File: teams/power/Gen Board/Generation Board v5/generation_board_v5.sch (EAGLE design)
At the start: 210 parts, among them U2 LT3652, U3 LT3652, U4 LT3652, U5 TPS732XX, U7 TPS732XX

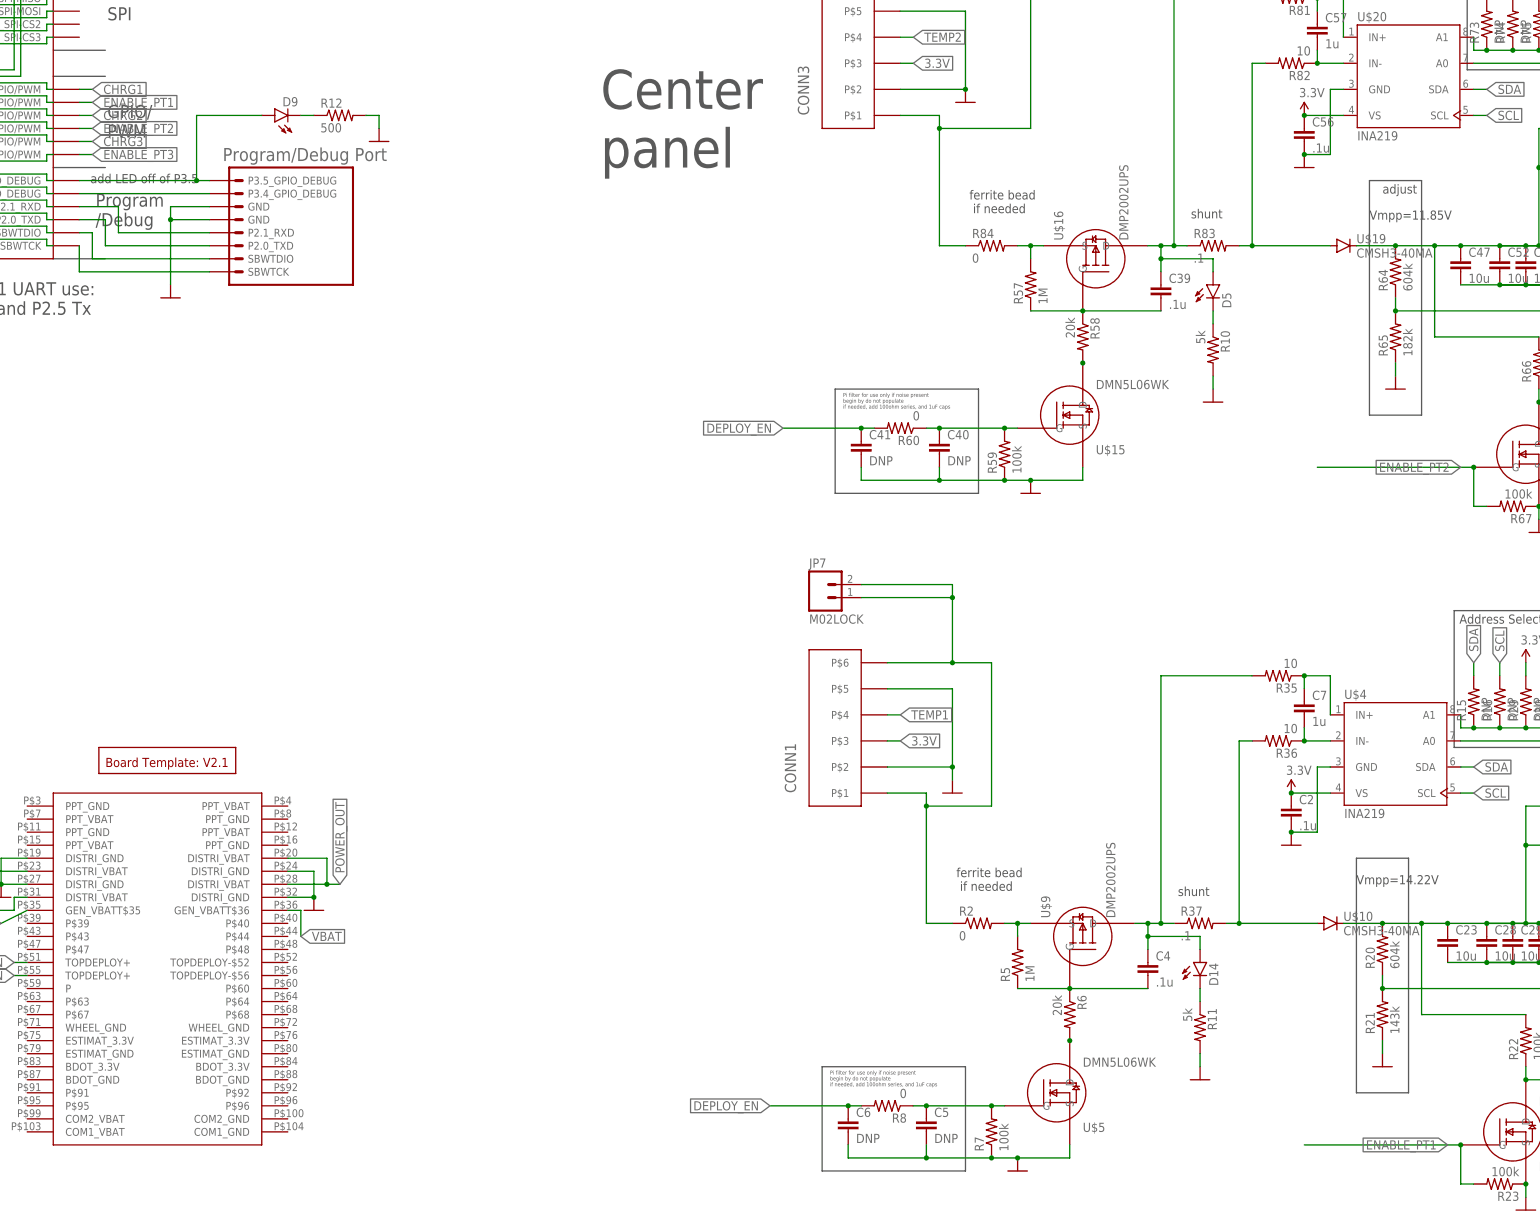
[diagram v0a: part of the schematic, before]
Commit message: minor changes
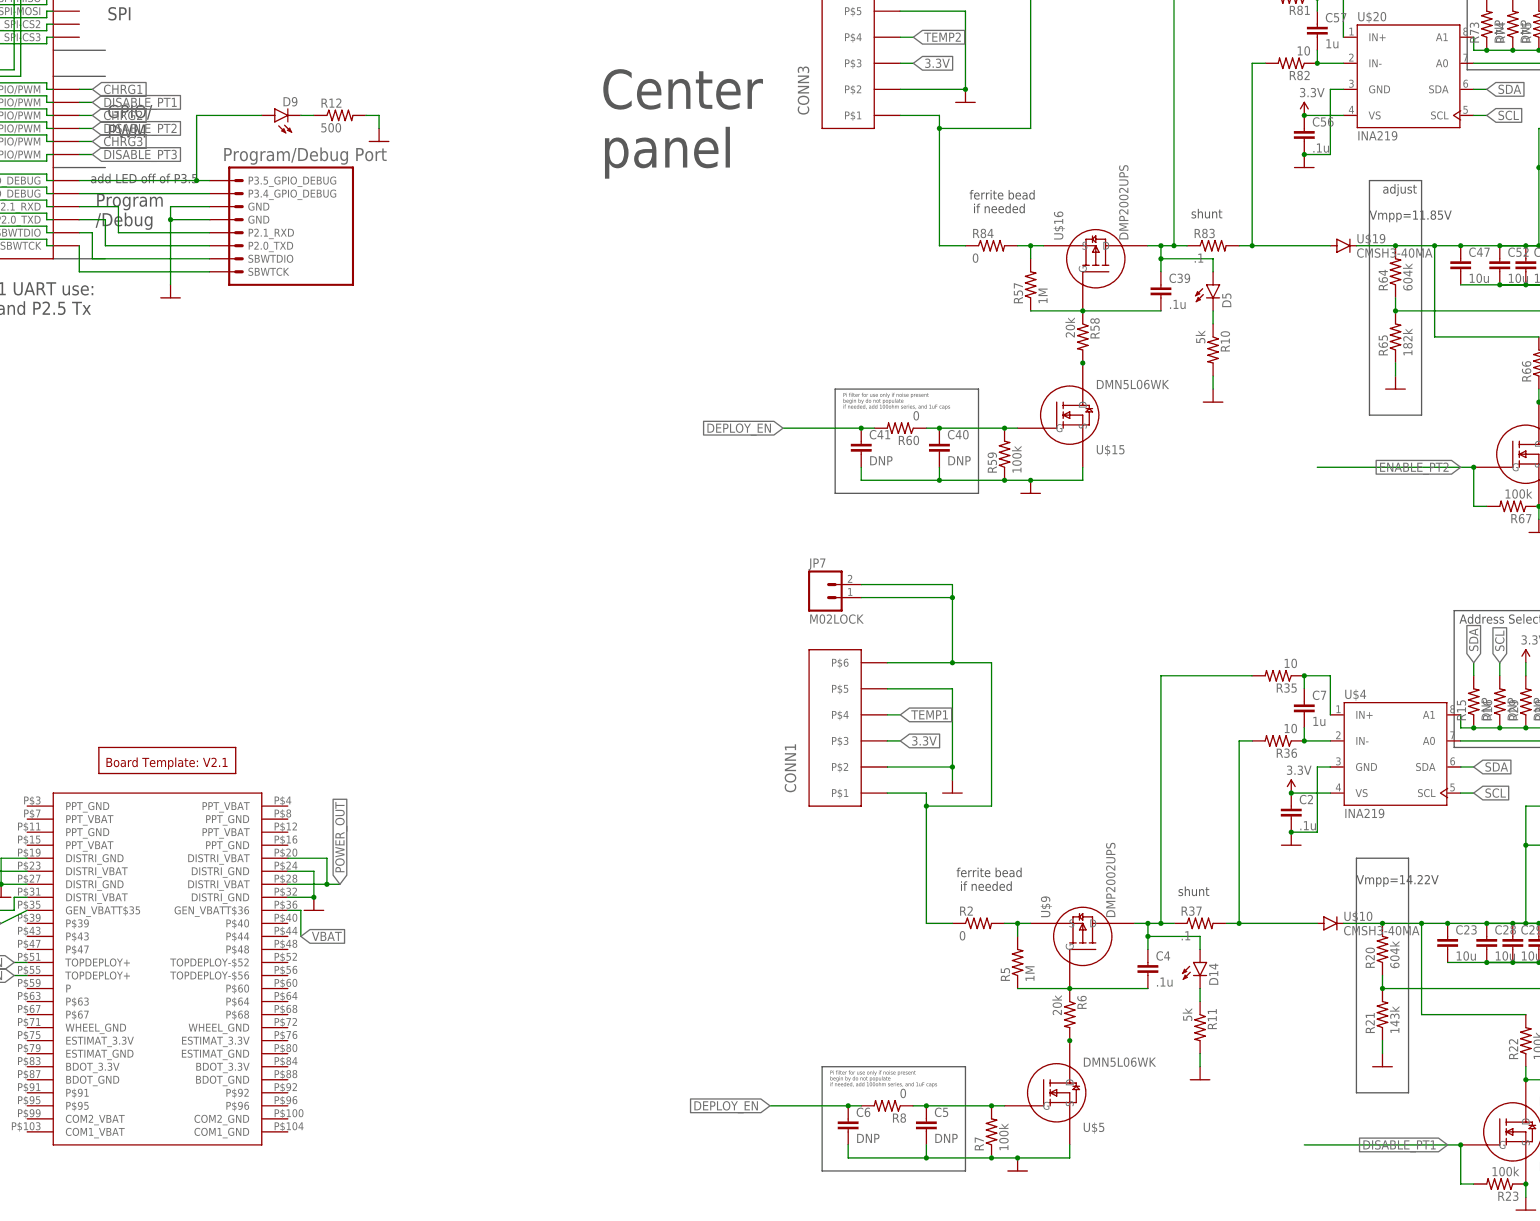
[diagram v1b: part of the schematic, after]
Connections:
- net ENABLE_PT1 renamed DISABLE_PT1
- new net DISABLE_PT2: BLK1.P3.6_GPIO/PWM
- new net DISABLE_PT3: BLK1.P2.6_GPIO/PWM
- net ENABLE_PT2: no longer BLK1.P3.6_GPIO/PWM
- net ENABLE_PT3: no longer BLK1.P2.6_GPIO/PWM
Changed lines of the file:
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@@
 </segment>
 </net>
-<net name="ENABLE_PT1" class="0">
+<net name="DISABLE_PT1" class="0">
 <segment>
 <pinref part="R23" gate="G$1" pin="2"/>
@@
 <junction x="185.42" y="223.52"/>
 </segment>
-<segment>
-<pinref part="BLK1" gate="G$1" pin="P3.6_GPIO/PWM"/>
-<wire x1="-86.36" y1="289.56" x2="-83.82" y2="289.56" width="0.1524" layer="91"/>
-<label x="-83.82" y="289.56" size="1.778" layer="95" xref="yes"/>
-</segment>
 </net>
 <net name="N$23" class="0">
@@
 <junction x="190.5" y="358.14"/>
 </segment>
-<segment>
-<pinref part="BLK1" gate="G$1" pin="P2.6_GPIO/PWM"/>
-<wire x1="-86.36" y1="284.48" x2="-83.82" y2="284.48" width="0.1524" layer="91"/>
-<label x="-83.82" y="284.48" size="1.778" layer="95" xref="yes"/>
-</segment>
 </net>
 <net name="N$32" class="0">
@@
 </segment>
 </net>
+<net name="DISABLE_PT2" class="0">
+<segment>
+<pinref part="BLK1" gate="G$1" pin="P3.6_GPIO/PWM"/>
+<wire x1="-86.36" y1="289.56" x2="-83.82" y2="289.56" width="0.1524" layer="91"/>
+<label x="-83.82" y="289.56" size="1.778" layer="95" xref="yes"/>
+</segment>
+</net>
+<net name="DISABLE_PT3" class="0">
+<segment>
+<pinref part="BLK1" gate="G$1" pin="P2.6_GPIO/PWM"/>
+<wire x1="-86.36" y1="284.48" x2="-83.82" y2="284.48" width="0.1524" layer="91"/>
+<label x="-83.82" y="284.48" size="1.778" layer="95" xref="yes"/>
+</segment>
+</net>
